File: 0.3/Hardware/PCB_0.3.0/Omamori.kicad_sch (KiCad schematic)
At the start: 37 parts, among them J1 Conn_01x04_Female, J2 Conn_01x05_Female, J3 Conn_01x06_Female, J4 Conn_01x03_Female, U1 BQ25570, U2 ATtiny1626, U3 TS-1233

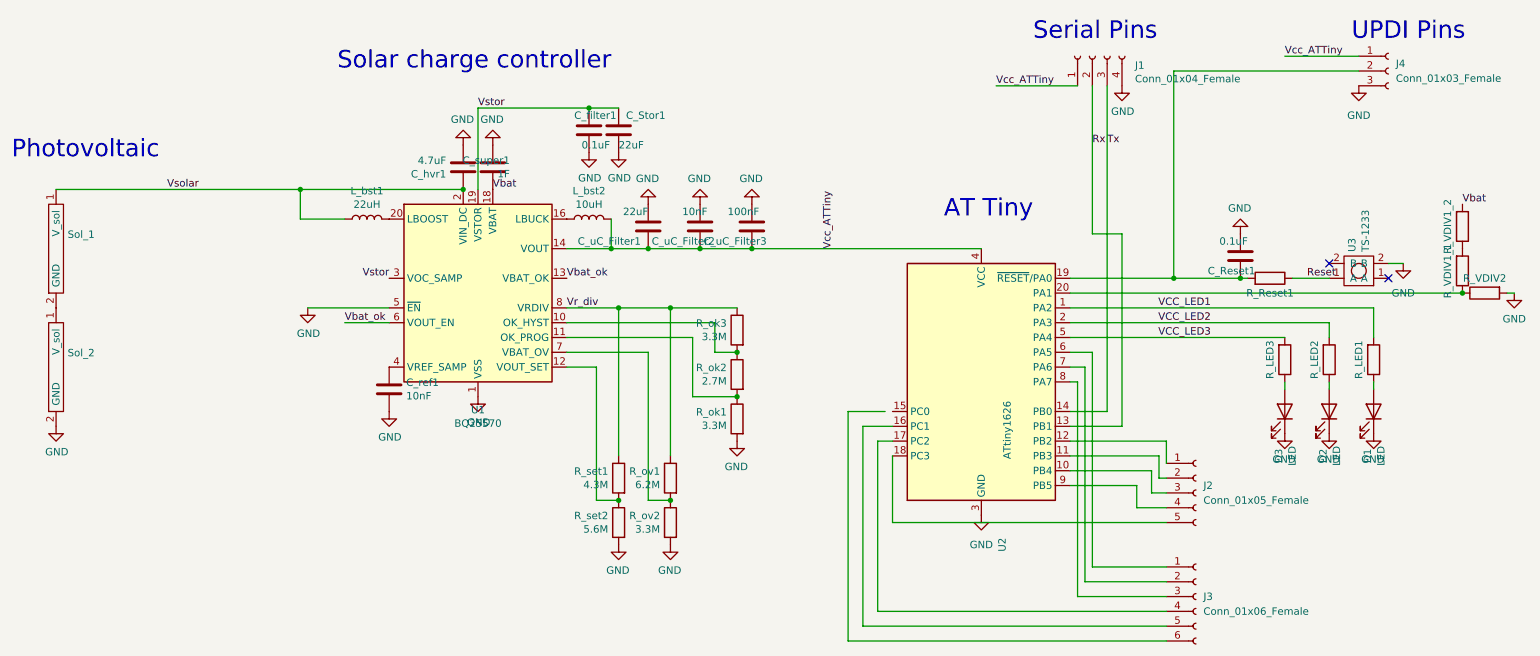
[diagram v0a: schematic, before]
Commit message: Temporarily finished pcb design.
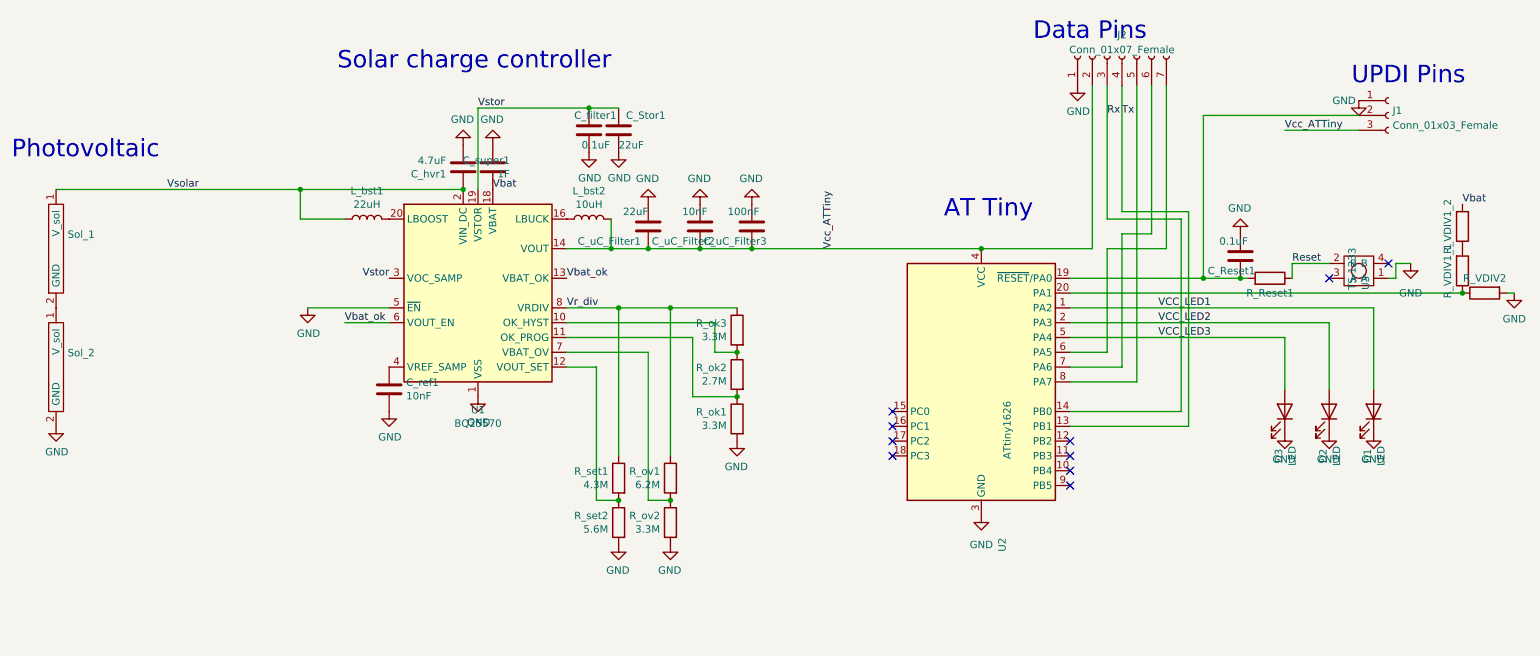
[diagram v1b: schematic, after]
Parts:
- removed J1: Conn_01x04_Female, Connector_PinHeader_1.27mm:PinHeader_1x04_P1.27mm_Horizontal, symbol Connector:Conn_01x04_Female
- removed J2: Conn_01x05_Female, Connector_PinHeader_2.54mm:PinHeader_1x05_P2.54mm_Vertical, symbol Connector:Conn_01x05_Female
- removed J3: Conn_01x06_Female, Connector_PinHeader_2.54mm:PinHeader_1x06_P2.54mm_Vertical, symbol Connector:Conn_01x06_Female
- removed R_LED1, R_LED3: 500, Resistor_SMD:R_0603_1608Metric_Pad0.98x0.95mm_HandSolder, symbol Device:R
- removed R_LED2: 500, Resistor_SMD:R_0603_1608Metric_Pad1.05x0.95mm_HandSolder, symbol Device:R
- added J2: Conn_01x07_Female, Connector_PinHeader_2.54mm:PinHeader_1x07_P2.54mm_Vertical, symbol Connector:Conn_01x07_Female
- renumbered J4 to J1
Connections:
- net GND: now also J1.1 (Pin_1), U3.1 (A), J2.1 (Pin_1); no longer J1.3 (Pin_3), U3.2 (B)
- net Reset: now also U3.2 (B); no longer U3.1 (A)
- net Rx: now also U2.14 (PB0), J2.3 (Pin_3); no longer U2.13 (PB1)
- net Tx: now also U2.13 (PB1), J2.4 (Pin_4); no longer U2.14 (PB0)
- net VCC_LED1: now also D1.2 (A)
- net VCC_LED2: now also D2.2 (A)
- net VCC_LED3: now also D3.2 (A)
- net Vcc_ATTiny: now also J1.3 (Pin_3), J2.2 (Pin_2); no longer J1.1 (Pin_1)
- net at U2.6 (PA5): now also J2.7 (Pin_7)
- net at U2.7 (PA6): now also J2.6 (Pin_6)
- net at U2.8 (PA7): now also J2.5 (Pin_5)
- no-connect marks 2 -> 10
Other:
- note added: "Data Pins"
- note removed: "Serial Pins"
- moved on the sheet: J1
